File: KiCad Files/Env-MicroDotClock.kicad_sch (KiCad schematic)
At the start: 47 parts, among them IC1 IS31FL3730-QFLS2-TR, IC2 IS31FL3730-QFLS2-TR, IC3 IS31FL3730-QFLS2-TR, IC4 IS31FL3730-QFLS2-TR, M1 Dip-14 Socket, M2 Dip-14 Socket, M3 Dip-14 Socket, M4 Dip-14 Socket, M5 Dip-14 Socket, M6 Dip-14 Socket, M7 Dip-14 Socket, M8 Dip-14 Socket, Q1 2SC1815, SW1 SKRK, SW2 SKRK, SW3 SKRK, SW4 SKRK, U1 Raspberry Pi Pico, U3 DS3231M

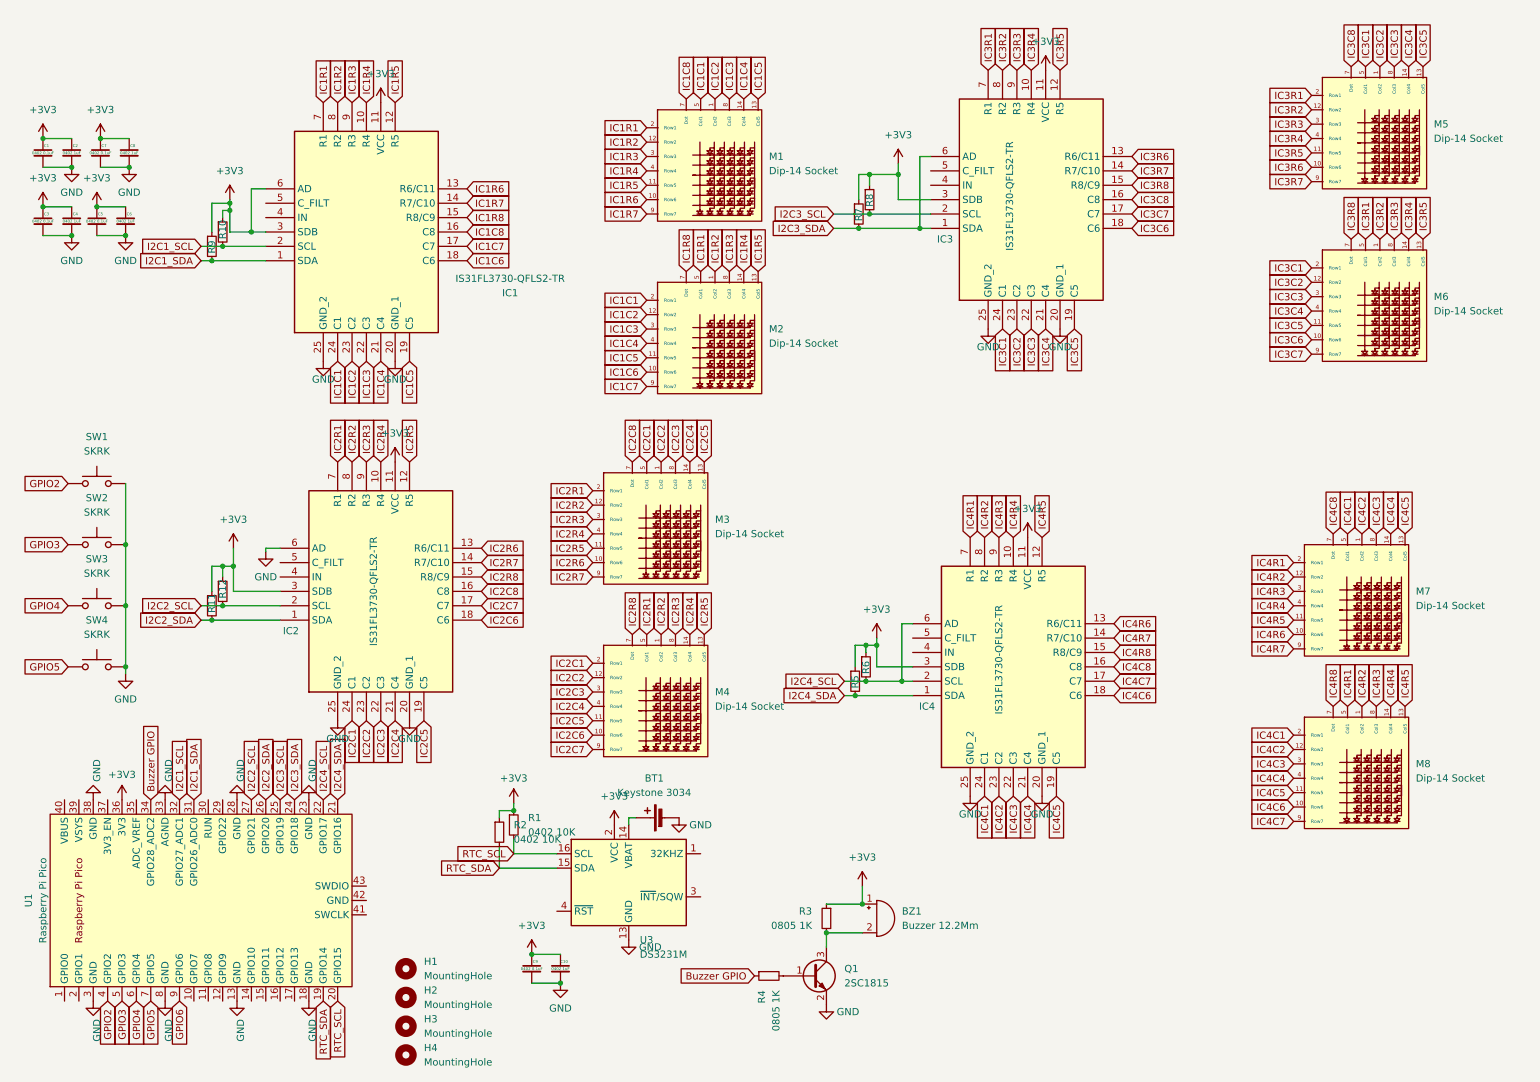
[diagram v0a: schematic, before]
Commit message: schema push
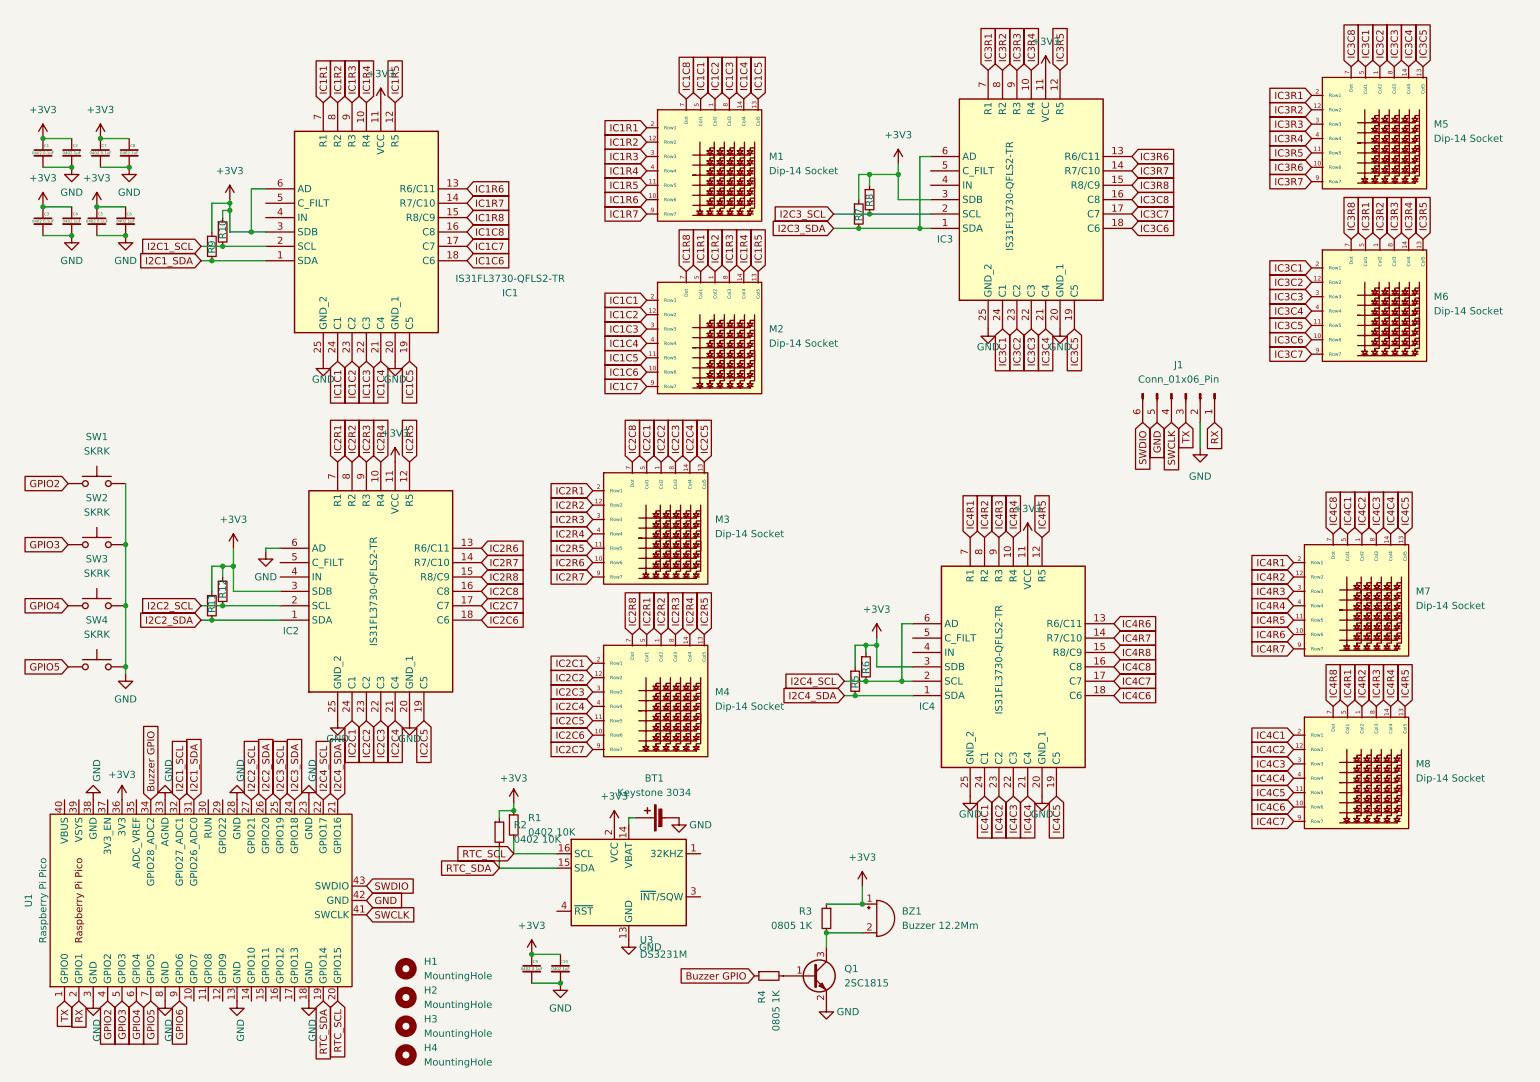
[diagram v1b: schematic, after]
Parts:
- added J1: Conn_01x06_Pin, Connector_PinHeader_2.54mm:PinHeader_1x06_P2.54mm_Vertical, symbol Connector:Conn_01x06_Pin
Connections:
- net GND: now also U1.42 (GND), J1.2 (Pin_2), J1.5 (Pin_5)
- net TX: now reaches U1.1 (GPIO0)
- net TX: now also J1.3 (Pin_3)
- net RX: now reaches U1.2 (GPIO1)
- net RX: now also J1.1 (Pin_1)
- net SWCLK: now reaches U1.41 (SWCLK)
- net SWCLK: now also J1.4 (Pin_4)
- net SWDIO: now reaches U1.43 (SWDIO)
- net SWDIO: now also J1.6 (Pin_6)
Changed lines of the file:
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@@
     (stroke (width 0) (type default))
   )
+  (wire (pts (xy 222.885 88.265) (xy 222.885 83.82))
+    (stroke (width 0) (type default))
+  )
   (wire (pts (xy 48.26 50.165) (xy 48.26 45.085))
     (stroke (width 0) (type default))
@@
     )
   )
+  (global_label "RX" (shape input) (at 225.425 83.82 270) (fields_autoplaced)
+    (effects (font (size 1.27 1.27)) (justify right))
+    (property "Intersheetrefs" "${INTERSHEET_REFS}" (at 225.425 89.2847 90)
+      (effects (font (size 1.27 1.27)) (justify right) hide)
+    )
+  )
   (global_label "IC2R2" (shape input) (at 115.57 98.425 180) (fields_autoplaced)
     (effects (font (size 1.27 1.27)) (justify right))
@@
     )
   )
+  (global_label "SWCLK" (shape input) (at 217.805 83.82 270) (fields_autoplaced)
+    (effects (font (size 1.27 1.27)) (justify right))
+    (property "Intersheetrefs" "${INTERSHEET_REFS}" (at 217.805 93.0342 90)
+      (effects (font (size 1.27 1.27)) (justify right) hide)
+    )
+  )
   (global_label "IC2C3" (shape input) (at 130.175 90.805 90) (fields_autoplaced)
     (effects (font (size 1.27 1.27)) (justify left))
@@
     )
   )
+  (global_label "SWDIO" (shape input) (at 212.725 83.82 270) (fields_autoplaced)
+    (effects (font (size 1.27 1.27)) (justify right))
+    (property "Intersheetrefs" "${INTERSHEET_REFS}" (at 212.725 92.6714 90)
+      (effects (font (size 1.27 1.27)) (justify right) hide)
+    )
+  )
+  (global_label "GND" (shape input) (at 75.565 168.275 0) (fields_autoplaced)
+    (effects (font (size 1.27 1.27)) (justify left))
+    (property "Intersheetrefs" "${INTERSHEET_REFS}" (at 82.4207 168.275 0)
+      (effects (font (size 1.27 1.27)) (justify left) hide)
+    )
+  )
   (global_label "IC1C1" (shape input) (at 134.62 26.67 90) (fields_autoplaced)
     (effects (font (size 1.27 1.27)) (justify left))
@@
     )
   )
+  (global_label "SWCLK" (shape input) (at 75.565 170.815 0) (fields_autoplaced)
+    (effects (font (size 1.27 1.27)) (justify left))
+    (property "Intersheetrefs" "${INTERSHEET_REFS}" (at 84.7792 170.815 0)
+      (effects (font (size 1.27 1.27)) (justify left) hide)
+    )
+  )
   (global_label "IC4R7" (shape input) (at 207.645 121.92 0) (fields_autoplaced)
     (effects (font (size 1.27 1.27)) (justify left))
@@
     )
   )
+  (global_label "TX" (shape input) (at 220.345 83.82 270) (fields_autoplaced)
+    (effects (font (size 1.27 1.27)) (justify right))
+    (property "Intersheetrefs" "${INTERSHEET_REFS}" (at 220.345 88.9823 90)
+      (effects (font (size 1.27 1.27)) (justify right) hide)
+    )
+  )
   (global_label "IC2R3" (shape input) (at 115.57 100.965 180) (fields_autoplaced)
     (effects (font (size 1.27 1.27)) (justify right))
@@
     )
   )
+  (global_label "RX" (shape input) (at 24.765 186.055 270) (fields_autoplaced)
+    (effects (font (size 1.27 1.27)) (justify right))
+    (property "Intersheetrefs" "${INTERSHEET_REFS}" (at 24.765 191.5197 90)
+      (effects (font (size 1.27 1.27)) (justify right) hide)
+    )
+  )
   (global_label "I2C2_SDA" (shape input) (at 46.355 118.745 180) (fields_autoplaced)
     (effects (font (size 1.27 1.27)) (justify right))
@@
     )
   )
+  (global_label "GND" (shape input) (at 215.265 83.82 270) (fields_autoplaced)
+    (effects (font (size 1.27 1.27)) (justify right))
+    (property "Intersheetrefs" "${INTERSHEET_REFS}" (at 215.265 90.6757 90)
+      (effects (font (size 1.27 1.27)) (justify right) hide)
+    )
+  )
   (global_label "IC3R1" (shape input) (at 252.095 51.435 90) (fields_autoplaced)
     (effects (font (size 1.27 1.27)) (justify left))
@@
     )
   )
+  (global_label "TX" (shape input) (at 22.225 186.055 270) (fields_autoplaced)
+    (effects (font (size 1.27 1.27)) (justify right))
+    (property "Intersheetrefs" "${INTERSHEET_REFS}" (at 22.225 191.2173 90)
+      (effects (font (size 1.27 1.27)) (justify right) hide)
+    )
+  )
   (global_label "I2C3_SDA" (shape input) (at 62.865 150.495 90) (fields_autoplaced)
     (effects (font (size 1.27 1.27)) (justify left))
@@
     )
   )
+  (global_label "SWDIO" (shape input) (at 75.565 165.735 0) (fields_autoplaced)
+    (effects (font (size 1.27 1.27)) (justify left))
+    (property "Intersheetrefs" "${INTERSHEET_REFS}" (at 84.4164 165.735 0)
+      (effects (font (size 1.27 1.27)) (justify left) hide)
+    )
+  )
   (global_label "IC2R6" (shape input) (at 95.885 106.045 0) (fields_autoplaced)
     (effects (font (size 1.27 1.27)) (justify left))
@@
     )
   )
+  (symbol (lib_id "power:GND") (at 222.885 88.265 0) (mirror y) (unit 1)
+    (in_bom yes) (on_board yes) (dnp no) (fields_autoplaced)
+    (property "Reference" "#PWR026" (at 222.885 94.615 0)
+      (effects (font (size 1.27 1.27)) hide)
+    )
+    (property "Value" "GND" (at 222.885 93.345 0)
+      (effects (font (size 1.27 1.27)))
+    )
+    (property "Footprint" "" (at 222.885 88.265 0)
+      (effects (font (size 1.27 1.27)) hide)
+    )
+    (property "Datasheet" "" (at 222.885 88.265 0)
+      (effects (font (size 1.27 1.27)) hide)
+    )
+    (pin "1")
+    (instances
+      (project "Env-MicroDotClock"
+        (path "/3dbeb8d8-208e-4f6d-8d30-b14372f68a4f"
+          (reference "#PWR026") (unit 1)
+        )
+      )
+    )
+  )
   (symbol (lib_id "power:GND") (at 198.12 67.31 0) (mirror y) (unit 1)
     (in_bom yes) (on_board yes) (dnp no) (fields_autoplaced)
@@
         )
       )
+    )
+  )
+  (symbol (lib_id "Connector:Conn_01x06_Pin") (at 220.345 78.74 270) (unit 1)
+    (in_bom yes) (on_board yes) (dnp no) (fields_autoplaced)
+    (property "Reference" "J1" (at 219.075 73.66 90)
+      (effects (font (size 1.27 1.27)))
+    )
+    (property "Value" "Conn_01x06_Pin" (at 219.075 76.2 90)
+      (effects (font (size 1.27 1.27)))
+    )
+    (property "Footprint" "Connector_PinHeader_2.54mm:PinHeader_1x06_P2.54mm_Vertical" (at 220.345 78.74 0)
+      (effects (font (size 1.27 1.27)) hide)
+    )
+    (property "Datasheet" "~" (at 220.345 78.74 0)
+      (effects (font (size 1.27 1.27)) hide)
+    )
+    (pin "1")
+    (pin "2")
+    (pin "3")
+    (pin "4")
+    (pin "5")
+    (pin "6")
+    (instances
+      (project "Env-MicroDotClock"
+        (path "/3dbeb8d8-208e-4f6d-8d30-b14372f68a4f"
+          (reference "J1") (unit 1)
+        )
+      )
